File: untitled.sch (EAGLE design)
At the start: 10 parts, among them IC1 TL494CD, Q1 IRF740, Q2 IRF740

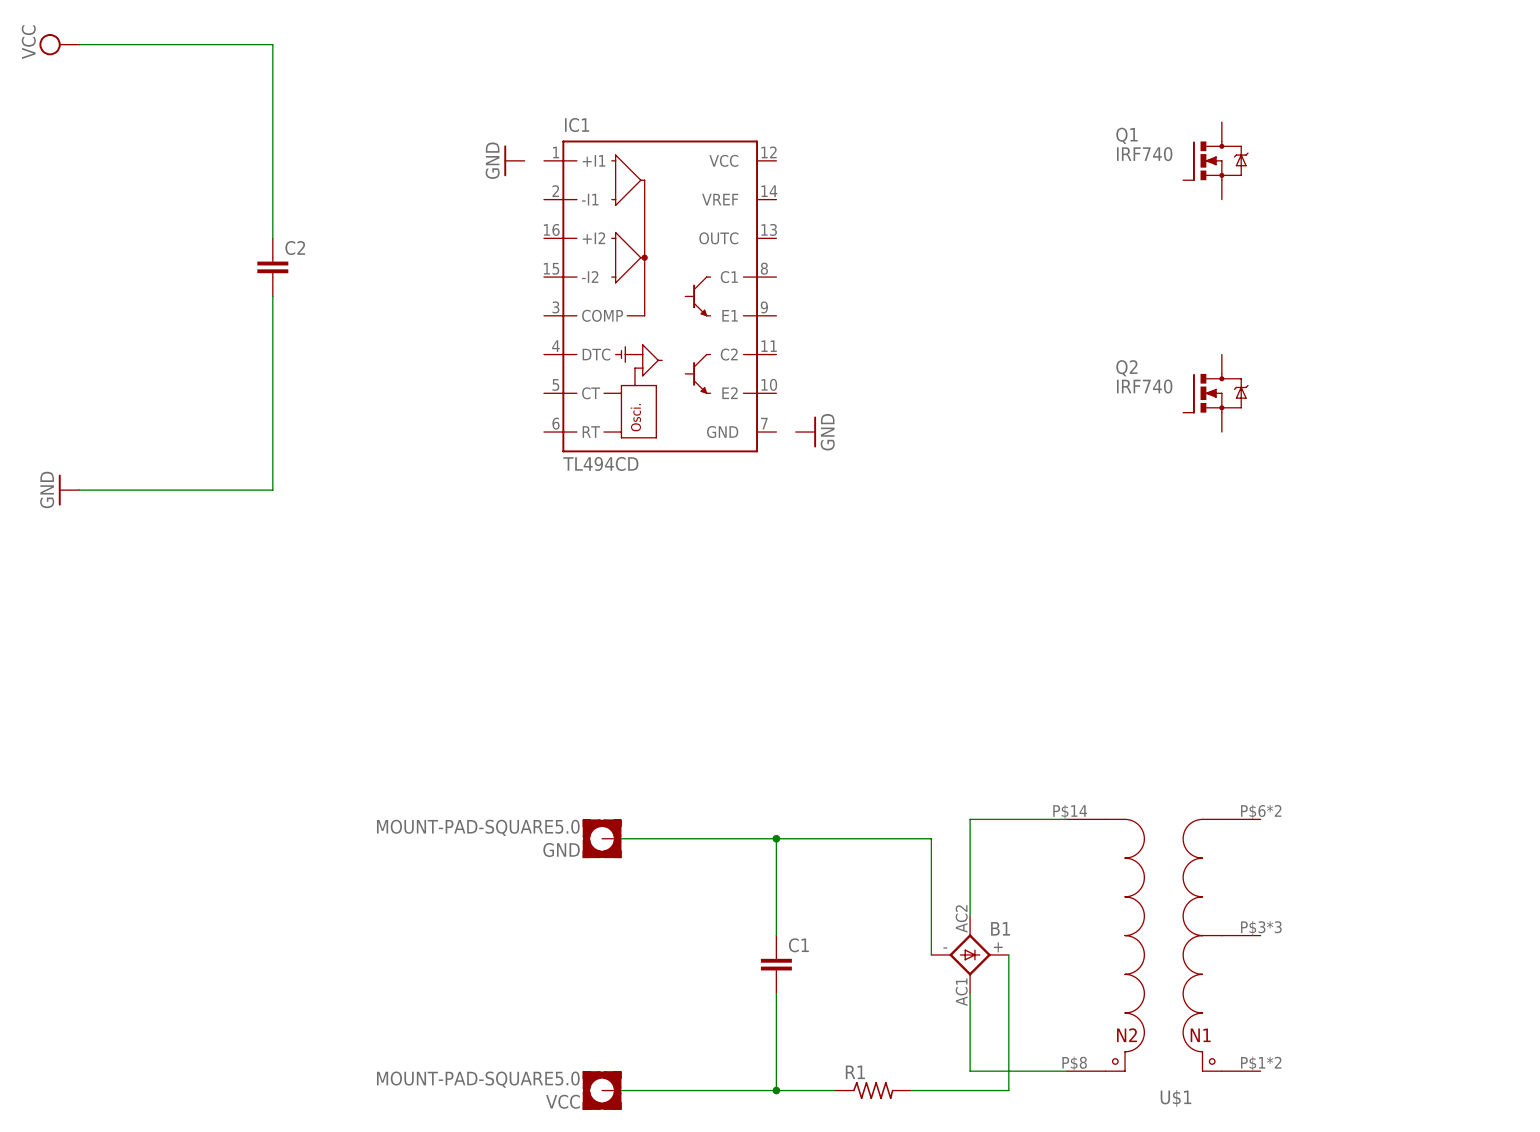
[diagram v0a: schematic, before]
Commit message: add
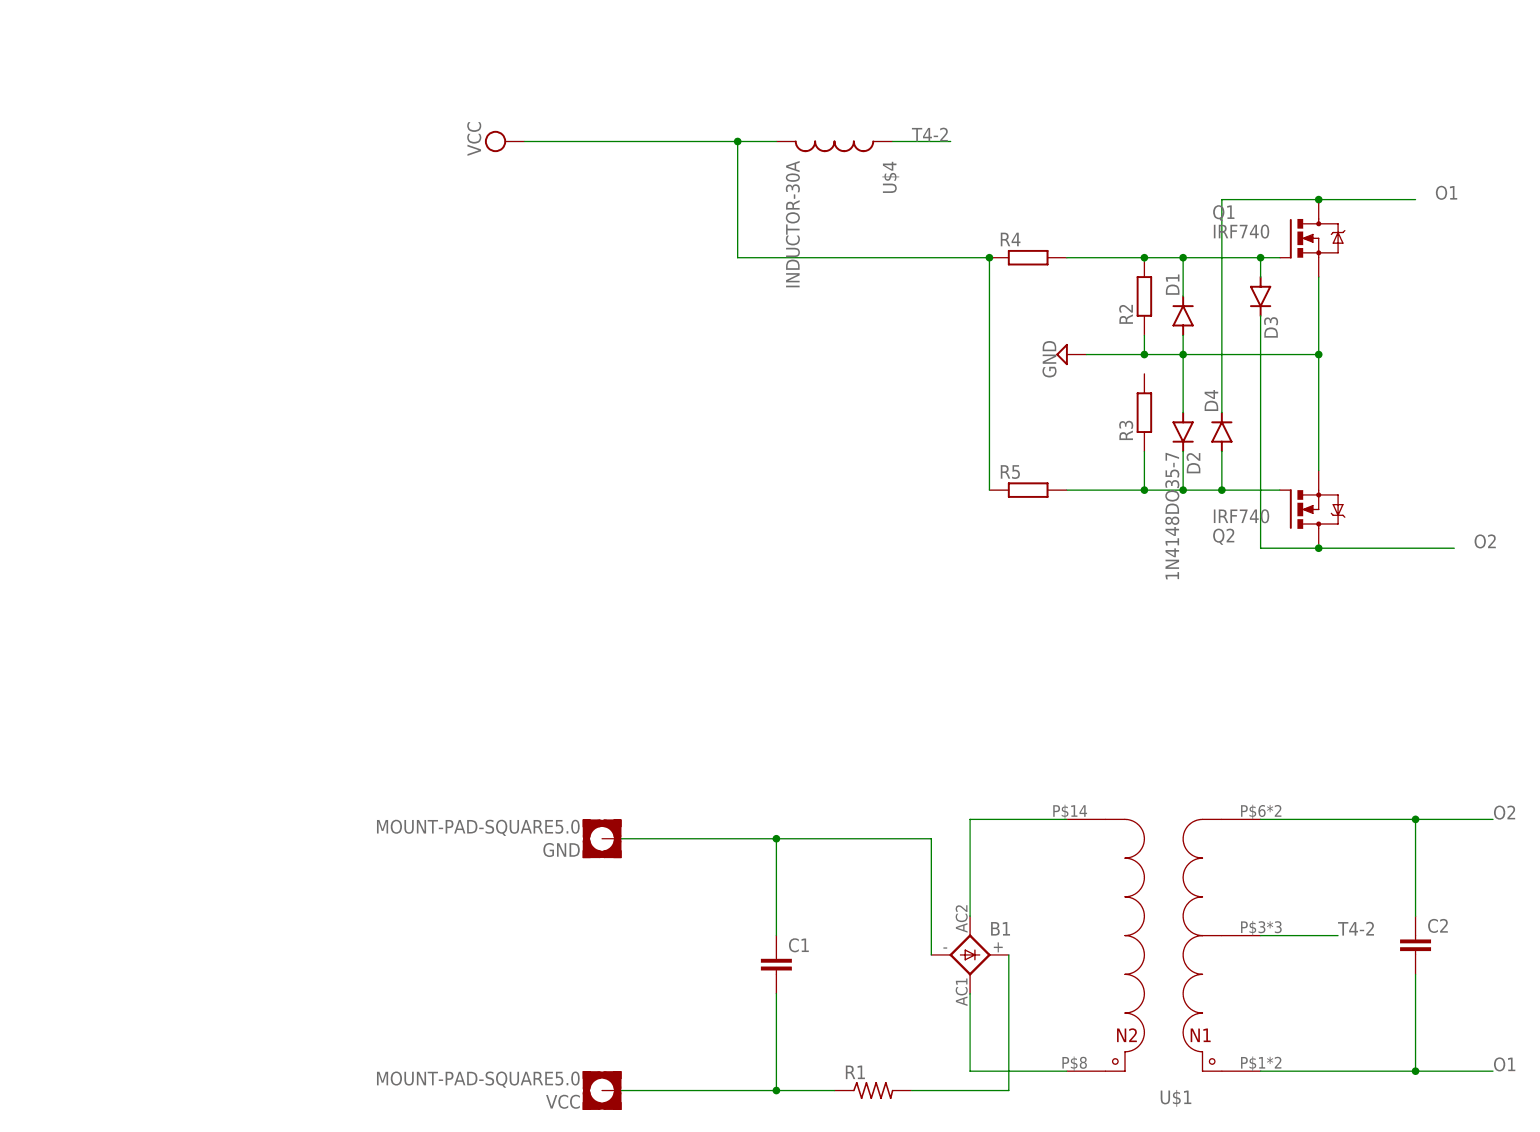
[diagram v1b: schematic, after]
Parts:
- removed IC1: TL494CD, linear:TL494CD
- added D1, D2: 1N4148DO35-7, diode:1N4148DO35-7
- added D3, D4: 1N4148DO35-10, diode:1N4148DO35-10
- added R2, R3, R4, R5: (no value), rcl:R-EU_0204/7
- added U$4: INDUCTOR-30A, untitled:INDUCTOR-30A
- C2: device capacitor-wima:C2.5/2 -> rcl:C-EU225-062X268
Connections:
- new net N$6: D1.C, D3.A, Q1.G, R2.2, R4.2
- new net N$7: D2.C, D4.A, Q2.G, R3.1, R5.2
- new net O1: C2.2, D4.C, Q1.D, U$1.T1
- new net O2: C2.1, D3.C, Q2.D, U$1.T3
- new net T4-2: U$1.T2, U$4.1
- net GND: now also D1.A, D2.A, Q1.S, Q2.S, R2.1; no longer C2.2
- net VCC: now also R4.1, R5.1, U$4.2; no longer C2.1
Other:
- moved on the sheet: C2, Q1, Q2
